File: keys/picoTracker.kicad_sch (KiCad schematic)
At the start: 15 parts, among them J1 Conn_01x10, SW1 LEFT, SW2 DOWN, SW3 RIGHT, SW4 UP, SW5 LT, SW6 B, SW7 A, SW8 RT, SW9 PLAY

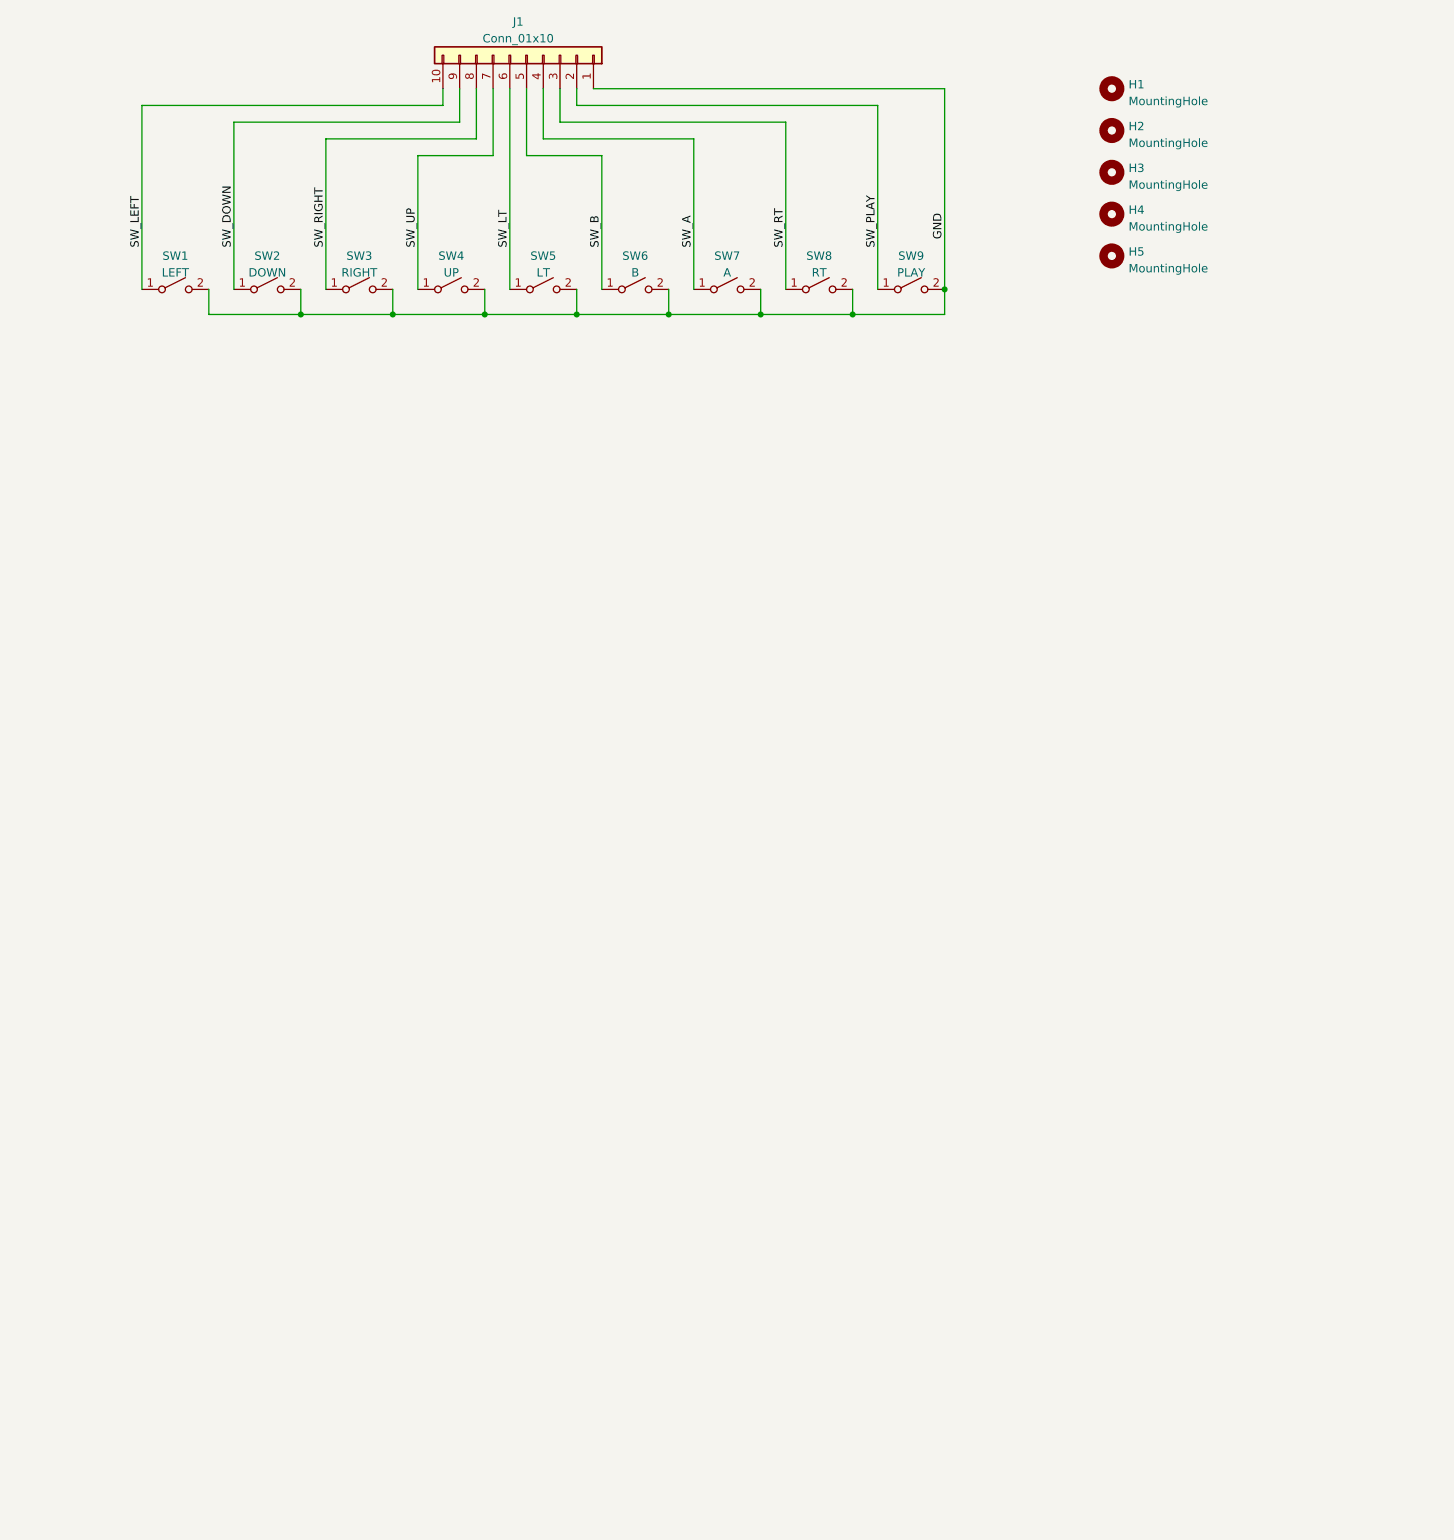
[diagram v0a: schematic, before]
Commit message: picoTracker PCB v2.1 and picoTrackerKeypad PCB v2.0
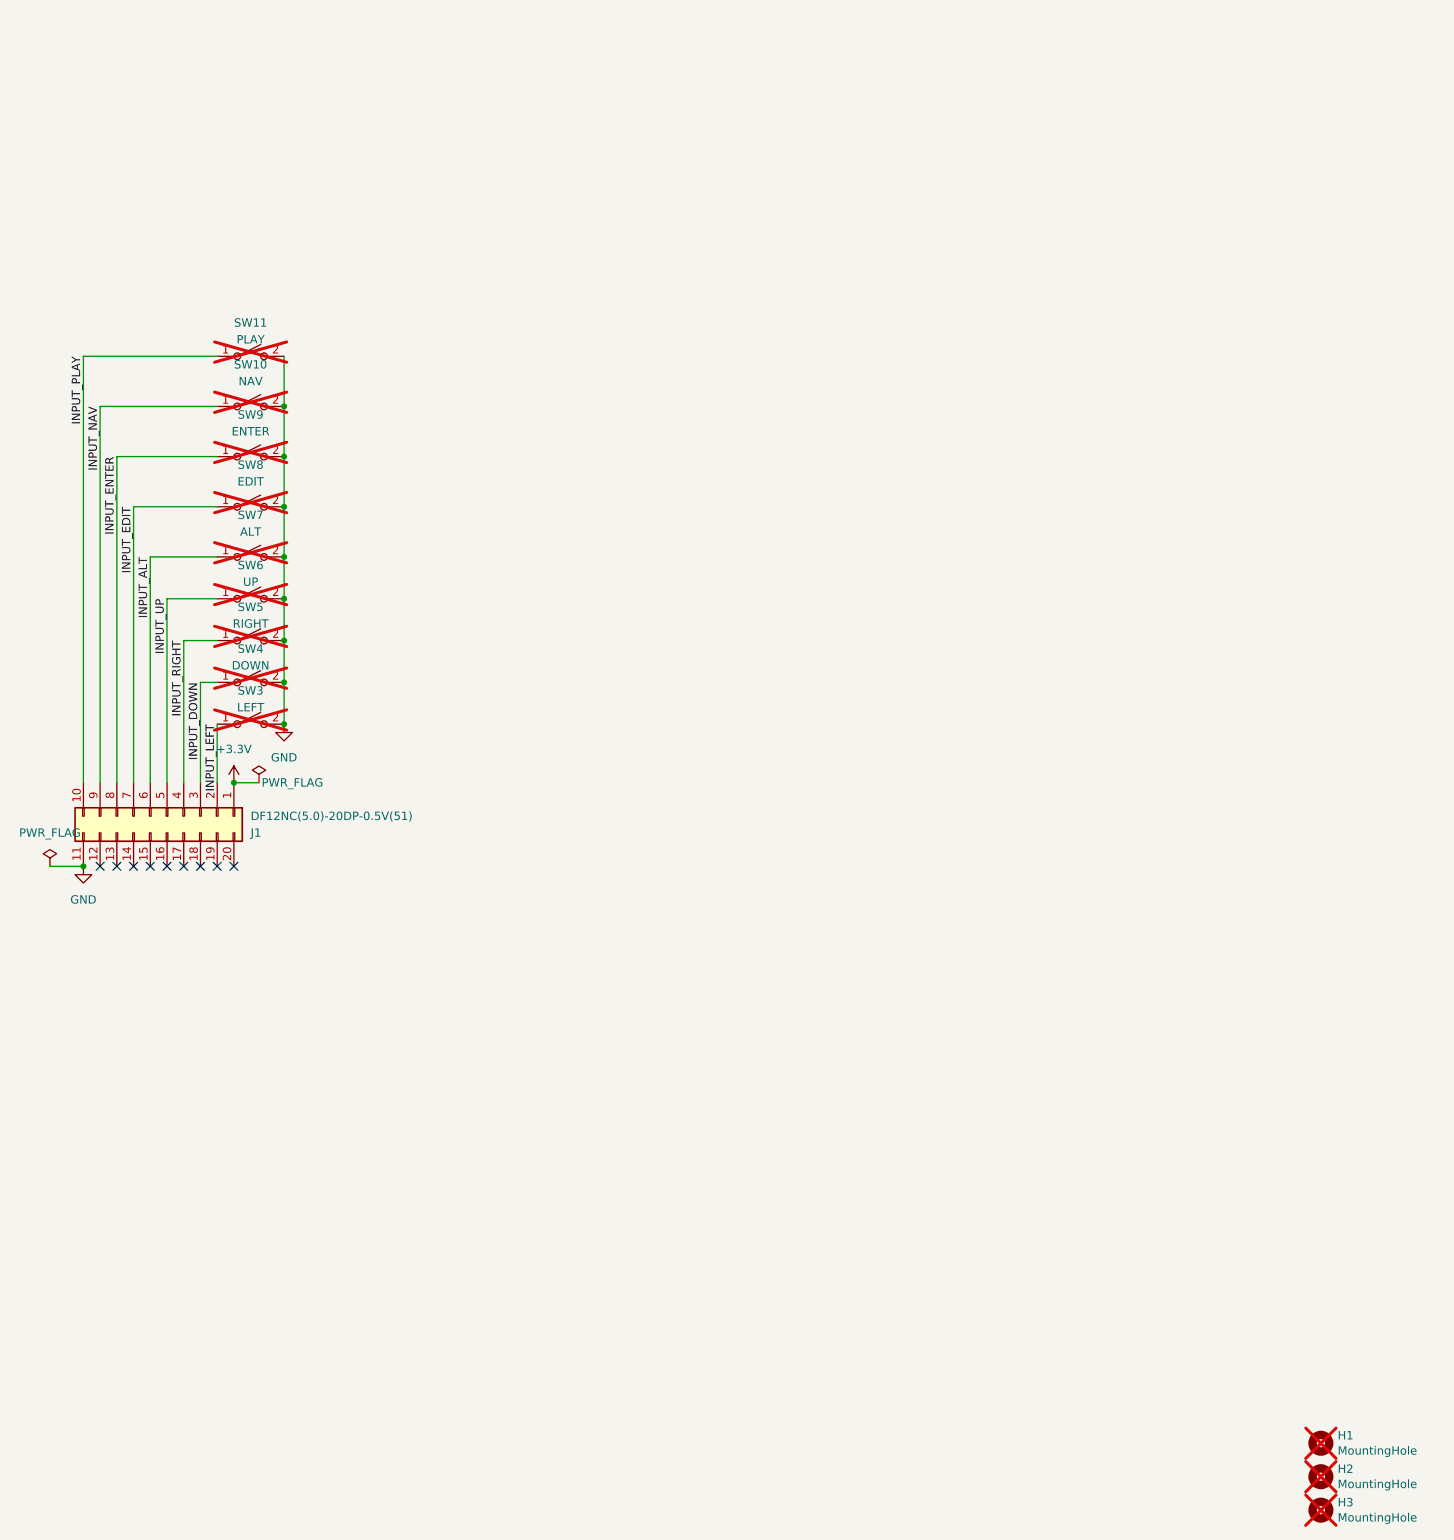
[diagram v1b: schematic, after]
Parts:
- removed H4, H5: MountingHole, MountingHole:MountingHole_2.2mm_M2, symbol Mechanical:MountingHole
- removed J1: Conn_01x10, Connector_PinHeader_2.54mm:PinHeader_1x10_P2.54mm_Vertical, symbol Connector_Generic:Conn_01x10
- removed SW1: LEFT, Cherry MX LP:Cherry-MX-Low-Profile, symbol Switch:SW_SPST
- removed SW2: DOWN, Cherry MX LP:Cherry-MX-Low-Profile, symbol Switch:SW_SPST
- added J1: DF12NC(5.0)-20DP-0.5V(51), Connector_Hirose:Hirose_DF12_DF12E3.0-20DP-0.5V_2x10_P0.50mm_Vertical, symbol Connector_Generic:Conn_02x10_Counter_Clockwise
- added SW10: NAV, project:Cherry-MX-Low-Profile-kailh, symbol Switch:SW_SPST
- added SW11: PLAY, project:Cherry-MX-Low-Profile-kailh, symbol Switch:SW_SPST
- H1, H2, H3: footprint MountingHole:MountingHole_2.2mm_M2 -> MountingHole:MountingHole_3.2mm_M3; now not fitted
- SW3: value RIGHT -> LEFT; footprint Cherry MX LP:Cherry-MX-Low-Profile -> project:Cherry-MX-Low-Profile-kailh; LCSC (none) -> C400229; now not fitted
- SW4: value UP -> DOWN; footprint Cherry MX LP:Cherry-MX-Low-Profile -> project:Cherry-MX-Low-Profile-kailh; LCSC (none) -> C400229; now not fitted
- SW5: value LT -> RIGHT; footprint Cherry MX LP:Cherry-MX-Low-Profile -> project:Cherry-MX-Low-Profile-kailh; LCSC (none) -> C400229; now not fitted
- SW6: value B -> UP; footprint Cherry MX LP:Cherry-MX-Low-Profile -> project:Cherry-MX-Low-Profile-kailh; LCSC (none) -> C400229; now not fitted
- SW7: value A -> ALT; footprint Cherry MX LP:Cherry-MX-Low-Profile -> project:Cherry-MX-Low-Profile-kailh; LCSC (none) -> C400229; now not fitted
- SW8: value RT -> EDIT; footprint Cherry MX LP:Cherry-MX-Low-Profile -> project:Cherry-MX-Low-Profile-kailh; LCSC (none) -> C400229; now not fitted
- SW9: value PLAY -> ENTER; footprint Cherry MX LP:Cherry-MX-Low-Profile -> project:Cherry-MX-Low-Profile-kailh; LCSC (none) -> C400229; now not fitted
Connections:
- net GND: now also J1.11 (Pin_11), SW10.2 (B), SW11.2 (B)
- net SW_A renamed INPUT_ALT
- net INPUT_ALT: now also J1.6 (Pin_6)
- net SW_B renamed INPUT_UP
- net INPUT_UP: now also J1.5 (Pin_5)
- net SW_LT renamed INPUT_RIGHT
- net INPUT_RIGHT: now also J1.4 (Pin_4)
- net SW_PLAY renamed INPUT_ENTER
- net INPUT_ENTER: now also J1.8 (Pin_8)
- net SW_RIGHT renamed INPUT_LEFT
- net INPUT_LEFT: now also J1.2 (Pin_2)
- net SW_RT renamed INPUT_EDIT
- net INPUT_EDIT: now also J1.7 (Pin_7)
- net SW_UP renamed INPUT_DOWN
- net INPUT_DOWN: now also J1.3 (Pin_3)
- new net +3.3V: J1.1 (Pin_1)
- new net INPUT_NAV: J1.9 (Pin_9), SW10.1 (A)
- new net INPUT_PLAY: J1.10 (Pin_10), SW11.1 (A)
- no-connect marks 0 -> 9
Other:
- title: picoTrackerPortable keys -> picoTracker
